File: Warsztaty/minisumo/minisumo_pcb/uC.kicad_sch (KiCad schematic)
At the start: 15 parts, among them U4 ATMEGA328P-AU, Y1 ECS-160-20-4DN

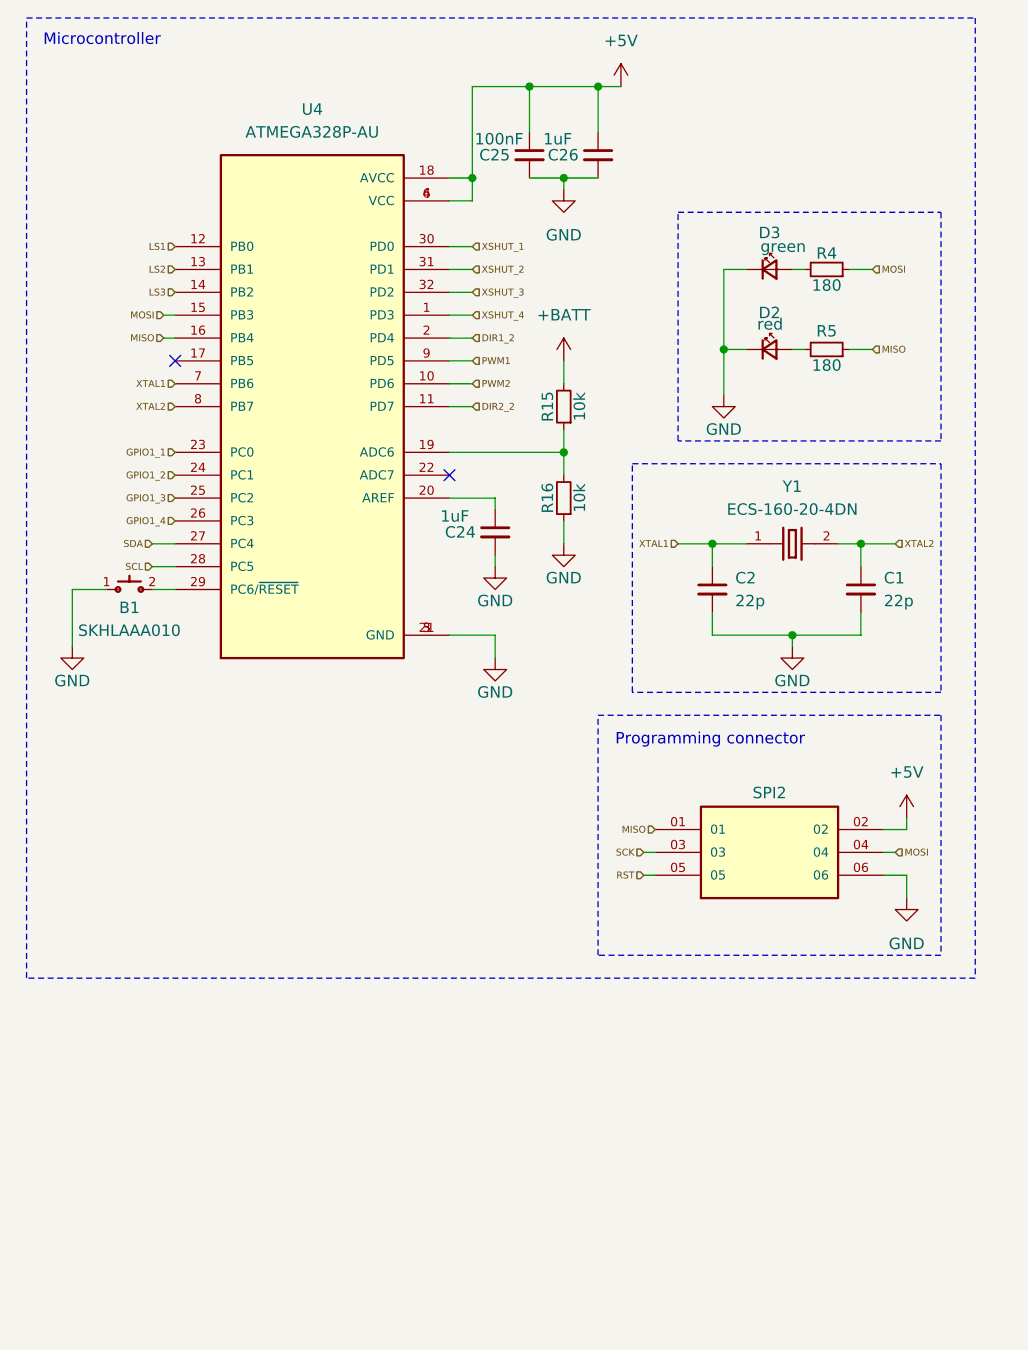
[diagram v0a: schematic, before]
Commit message: chyba gotowy schemat
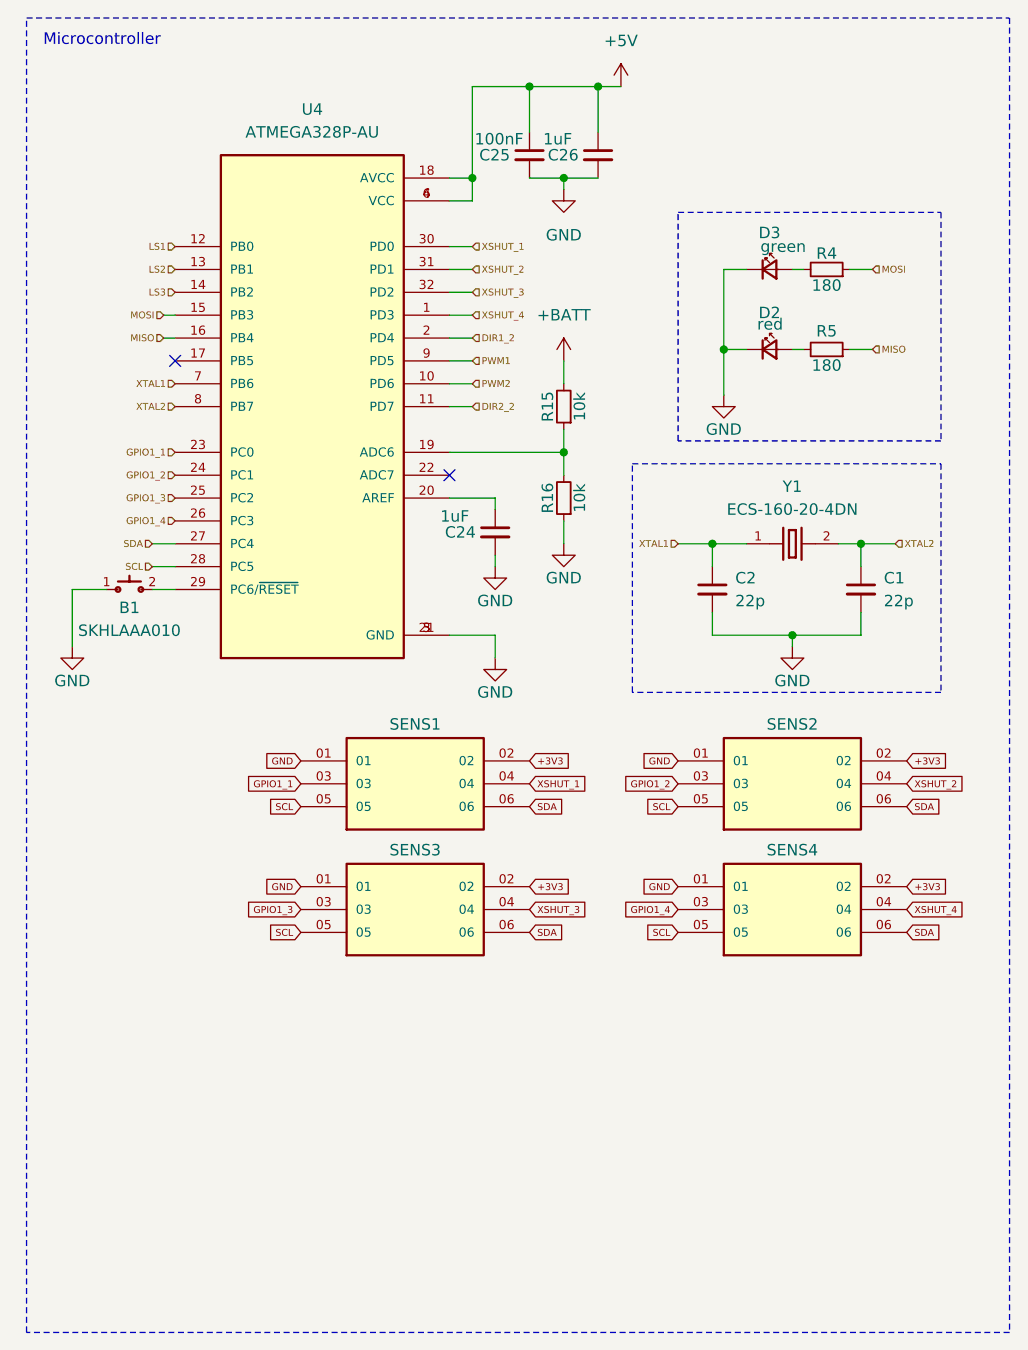
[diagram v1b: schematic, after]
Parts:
- removed SPI2: MTSW-103-23-F-D-230, MTSW-103-23-F-D-230:SAMTEC_MTSW-103-23-F-D-230, symbol MTSW-103-23-F-D-230:MTSW-103-23-F-D-230
- added SENS1, SENS2, SENS3, SENS4: MTSW-103-23-F-D-230, MTSW-103-23-F-D-230:SAMTEC_MTSW-103-23-F-D-230, symbol MTSW-103-23-F-D-230:MTSW-103-23-F-D-230
- C1, C2, C24, C25, C26: footprint (none) -> Capacitor_SMD:C_0805_2012Metric_Pad1.18x1.45mm_HandSolder
- D2, D3: footprint (none) -> LED_THT:LED_D3.0mm
- R15, R16, R4, R5: footprint (none) -> Resistor_SMD:R_0805_2012Metric_Pad1.20x1.40mm_HandSolder
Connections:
- net GND: now also SENS1.01, SENS2.01, SENS3.01, SENS4.01
- net GPIO1_1: now also SENS1.03
- net GPIO1_2: now also SENS2.03
- net GPIO1_3: now also SENS3.03
- net GPIO1_4: now also SENS4.03
- net SCL: now also SENS1.05, SENS2.05, SENS3.05, SENS4.05
- net SDA: now also SENS1.06, SENS2.06, SENS3.06, SENS4.06
- net XSHUT_1: now also SENS1.04
- net XSHUT_2: now also SENS2.04
- net XSHUT_3: now also SENS3.04
- net XSHUT_4: now also SENS4.04
- new net +3V3: SENS1.02, SENS2.02, SENS3.02, SENS4.02
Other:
- note removed: "Programming connector"

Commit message: chyba gotowy schemat
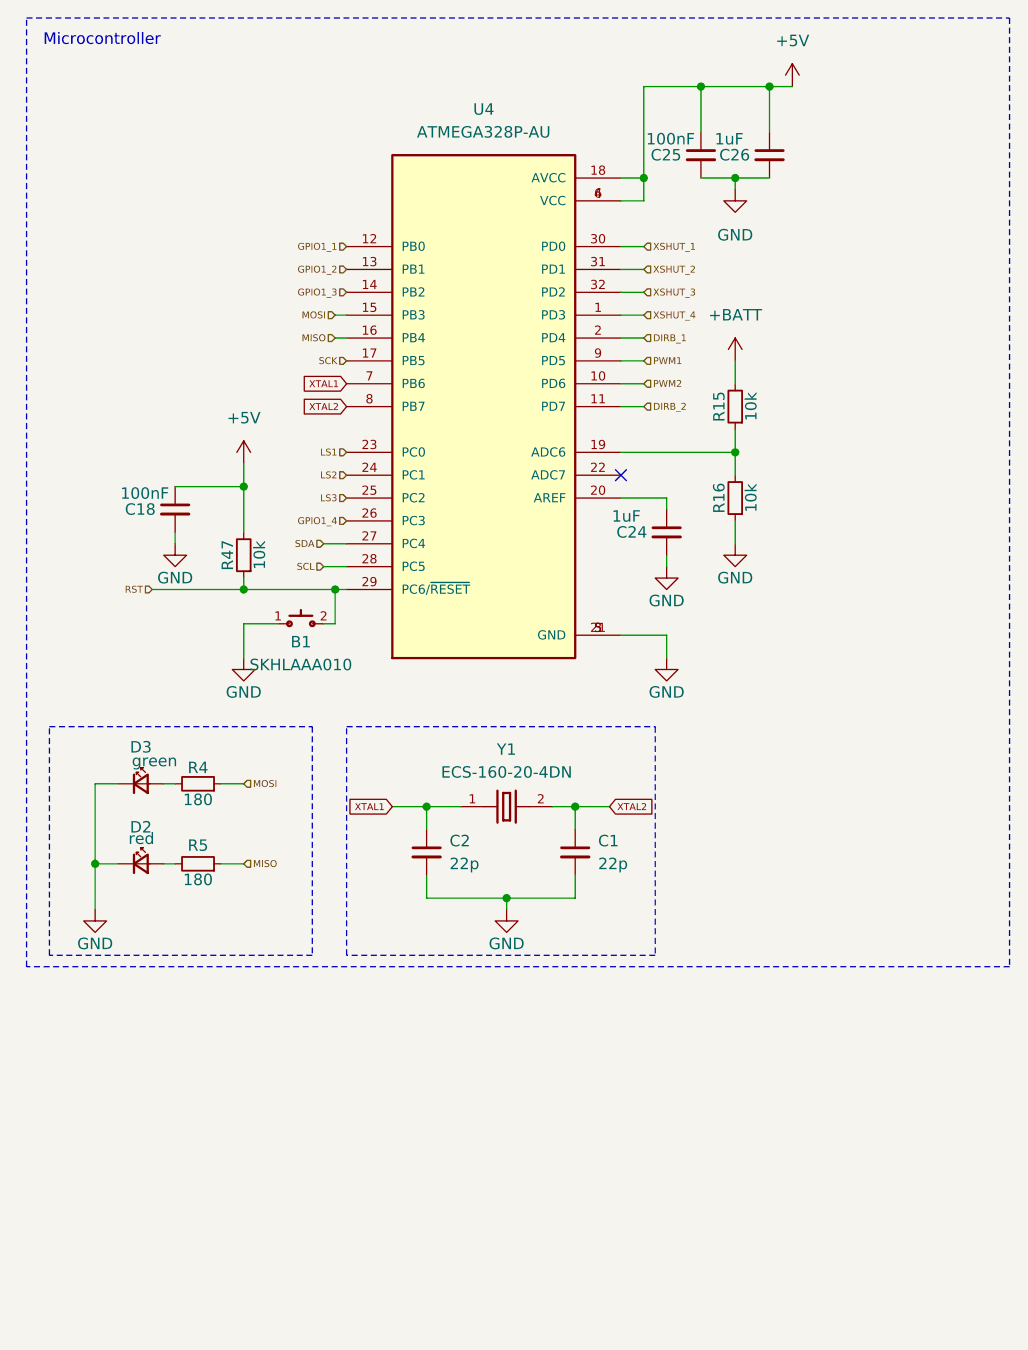
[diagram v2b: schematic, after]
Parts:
- removed SENS1, SENS2, SENS3, SENS4: MTSW-103-23-F-D-230, MTSW-103-23-F-D-230:SAMTEC_MTSW-103-23-F-D-230, symbol MTSW-103-23-F-D-230:MTSW-103-23-F-D-230
- added C18: 100nF, Capacitor_SMD:C_0805_2012Metric_Pad1.18x1.45mm_HandSolder, symbol Device:C_Small
- added R47: 10k, Resistor_SMD:R_0805_2012Metric_Pad1.20x1.40mm_HandSolder, symbol Device:R_Small
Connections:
- net +5V: now also C18.1, R47.2
- net GND: now also C18.2
- net GPIO1_1: now also U4.12 (PB0); no longer U4.23 (PC0)
- net GPIO1_2: now also U4.13 (PB1); no longer U4.24 (PC1)
- net GPIO1_3: now also U4.14 (PB2); no longer U4.25 (PC2)
- net LS1: now also U4.23 (PC0); no longer U4.12 (PB0)
- net LS2: now also U4.24 (PC1); no longer U4.13 (PB1)
- net LS3: now also U4.25 (PC2); no longer U4.14 (PB2)
- net SCK: now reaches U4.17 (PB5)
- net RST: now reaches B1.2, U4.29 (PC6/~{RESET})
- net RST: now also R47.1
- net DIR1_2 renamed DIRB_1
- net DIR2_2 renamed DIRB_2
- no-connect marks 2 -> 1
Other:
- moved on the sheet: B1, C1, C2, C24, C25, C26, D2, D3, R15, R16, R4, R5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
